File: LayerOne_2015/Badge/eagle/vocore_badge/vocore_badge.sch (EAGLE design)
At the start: 21 parts, among them U1 FT232RL-BASICSSOP

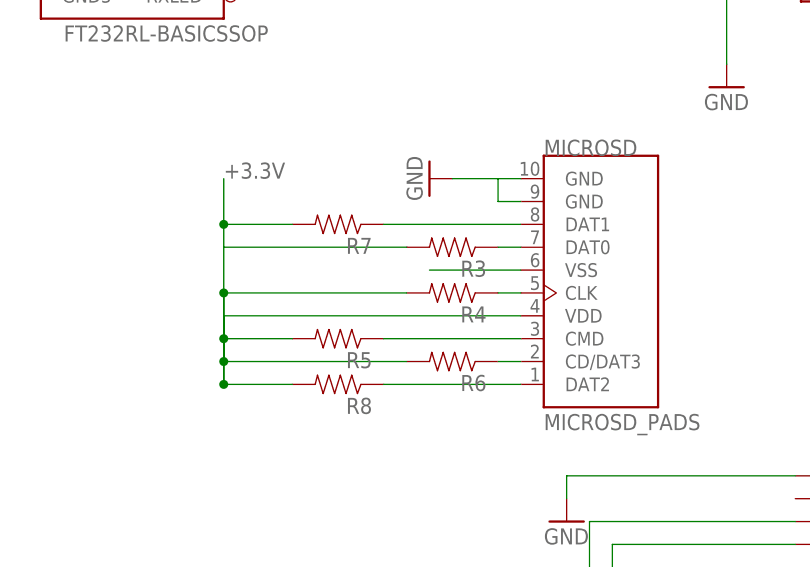
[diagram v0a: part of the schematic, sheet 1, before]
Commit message: 20k SDCARD
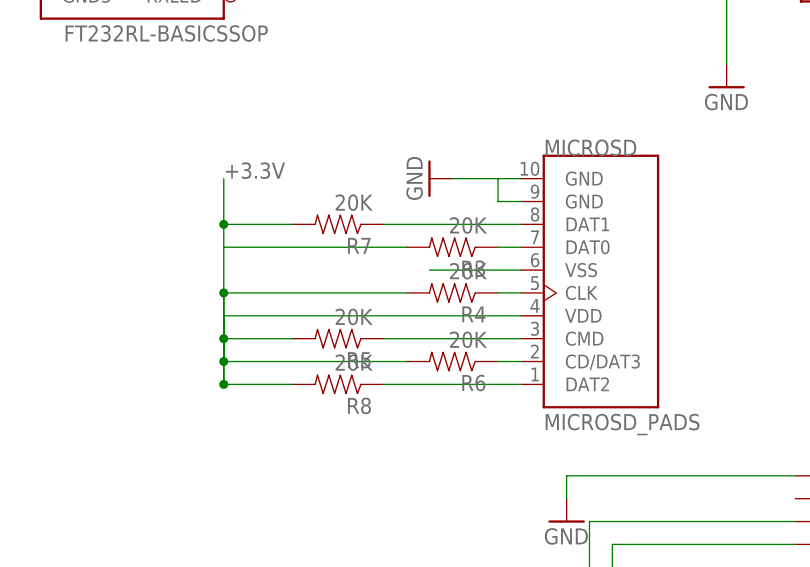
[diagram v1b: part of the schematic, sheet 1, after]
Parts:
- R3, R4, R5, R6, R7, R8: value (none) -> 20K
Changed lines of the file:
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@@
 <part name="R1" library="SparkFun-Resistors" deviceset="RESISTOR" device="0805-RES" value="150R"/>
 <part name="R2" library="SparkFun-Resistors" deviceset="RESISTOR" device="0805-RES" value="150"/>
-<part name="R3" library="SparkFun-Resistors" deviceset="RESISTOR" device="0805-RES"/>
-<part name="R4" library="SparkFun-Resistors" deviceset="RESISTOR" device="0805-RES"/>
-<part name="R5" library="SparkFun-Resistors" deviceset="RESISTOR" device="0805-RES"/>
-<part name="R6" library="SparkFun-Resistors" deviceset="RESISTOR" device="0805-RES"/>
-<part name="R7" library="SparkFun-Resistors" deviceset="RESISTOR" device="0805-RES"/>
-<part name="R8" library="SparkFun-Resistors" deviceset="RESISTOR" device="0805-RES"/>
+<part name="R3" library="SparkFun-Resistors" deviceset="RESISTOR" device="0805-RES" value="20K"/>
+<part name="R4" library="SparkFun-Resistors" deviceset="RESISTOR" device="0805-RES" value="20K"/>
+<part name="R5" library="SparkFun-Resistors" deviceset="RESISTOR" device="0805-RES" value="20K"/>
+<part name="R6" library="SparkFun-Resistors" deviceset="RESISTOR" device="0805-RES" value="20K"/>
+<part name="R7" library="SparkFun-Resistors" deviceset="RESISTOR" device="0805-RES" value="20K"/>
+<part name="R8" library="SparkFun-Resistors" deviceset="RESISTOR" device="0805-RES" value="20K"/>
 <part name="USB1" library="vocore_dock" deviceset="USB_MICRO_A" device="USB_MICRO_A" value="USB_MICRO_A"/>
 <part name="GND4" library="supply1" deviceset="GND" device=""/>
